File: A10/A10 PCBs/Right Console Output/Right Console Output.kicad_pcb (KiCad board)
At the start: 2 copper layers, 99.7 x 98.4 mm, 78 parts, among them J1 BACKLIGHT, J10 PATCH, J11 PATCH, J12 BACKLIGHT, J13 BACKLIGHT, J14 BACKLIGHT, J15 PATCH, J16 PATCH, J17 BACKLIGHT, J18 BACKLIGHT, J19 BACKLIGHT, J2 BACKLIGHT, J20 5VIN, J21 LOX, J22 12VIN, J23 CABIN_PRES, J24 PWM, J25 PWM, J26 Communication, J27 OXY_REG, J28 RIGHT FUEL, J29 LEFT_FUEL, J3 BACKLIGHT, J30 RIGHT_HYD, J31 LEFT_HYD, J32 Analog, J33 Analog, J34 CABIN_PRES, J35 OXY_REG, J36 LOX, J37 RIGHT_HYD, J38 LEFT_FUEL, J39 RIGHT FUEL, J4 BACKLIGHT, J40 LEFT_HYD, J41 Power, J42 Power, J43 Analog, J44 Analog, J45 Digital, J46 PWM, J47 PWM, J48 Communication, J49 CAUTION_UPPER_DIGIT, J5 BACKLIGHT, J50 CAUTION_UPPER_SEG, J51 CAUTION_LOW_DIGITS, J52 CAUTION_LOWER_SEG, J53 OXY_LED, J54 TACAN_TEST, J55 FORWARD_SEGEMENTS, J56 FORWARD_DIGITS, J6 BACKLIGHT, J7 BACKLIGHT, J8 BACKLIGHT, J9 BACKLIGHT, Q1 IRF1405PBF, U1 USR-ES1, U2 MAX7219-A, U3 MAX7219-B

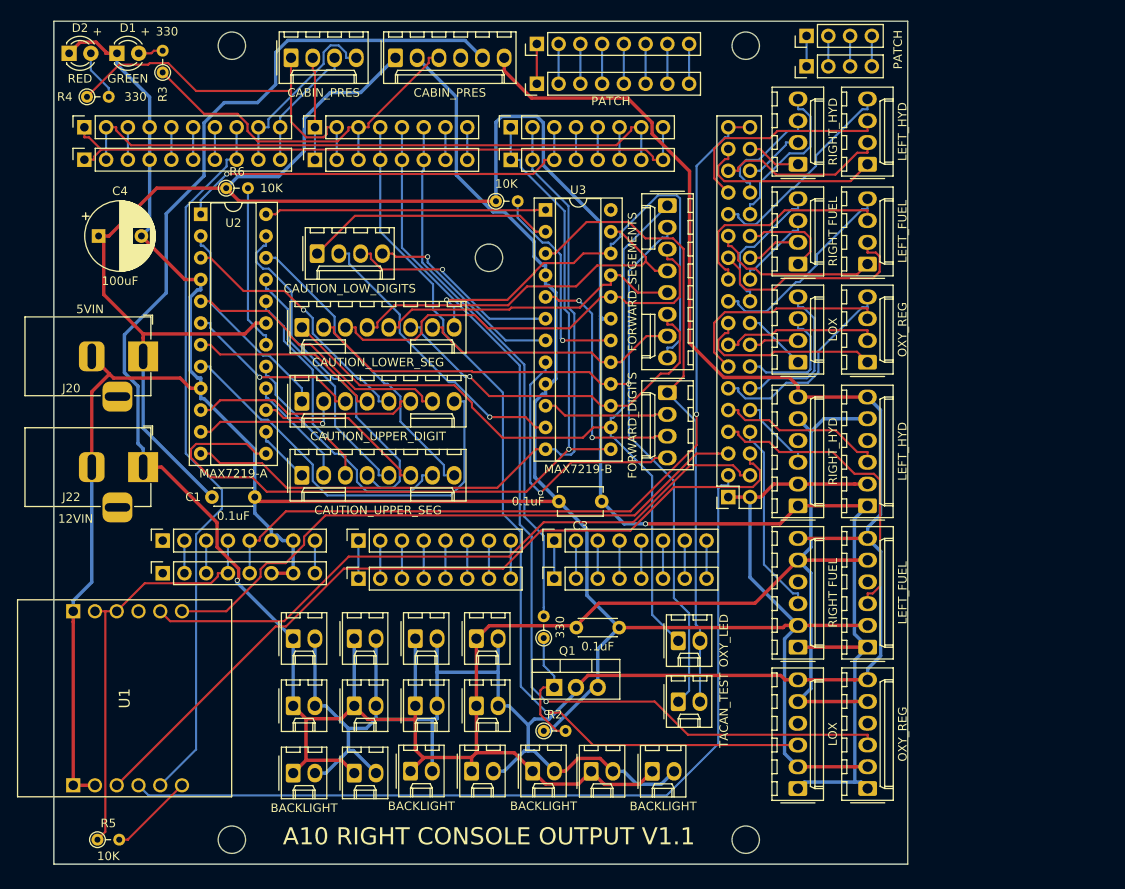
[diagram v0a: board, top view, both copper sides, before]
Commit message: a10 PC
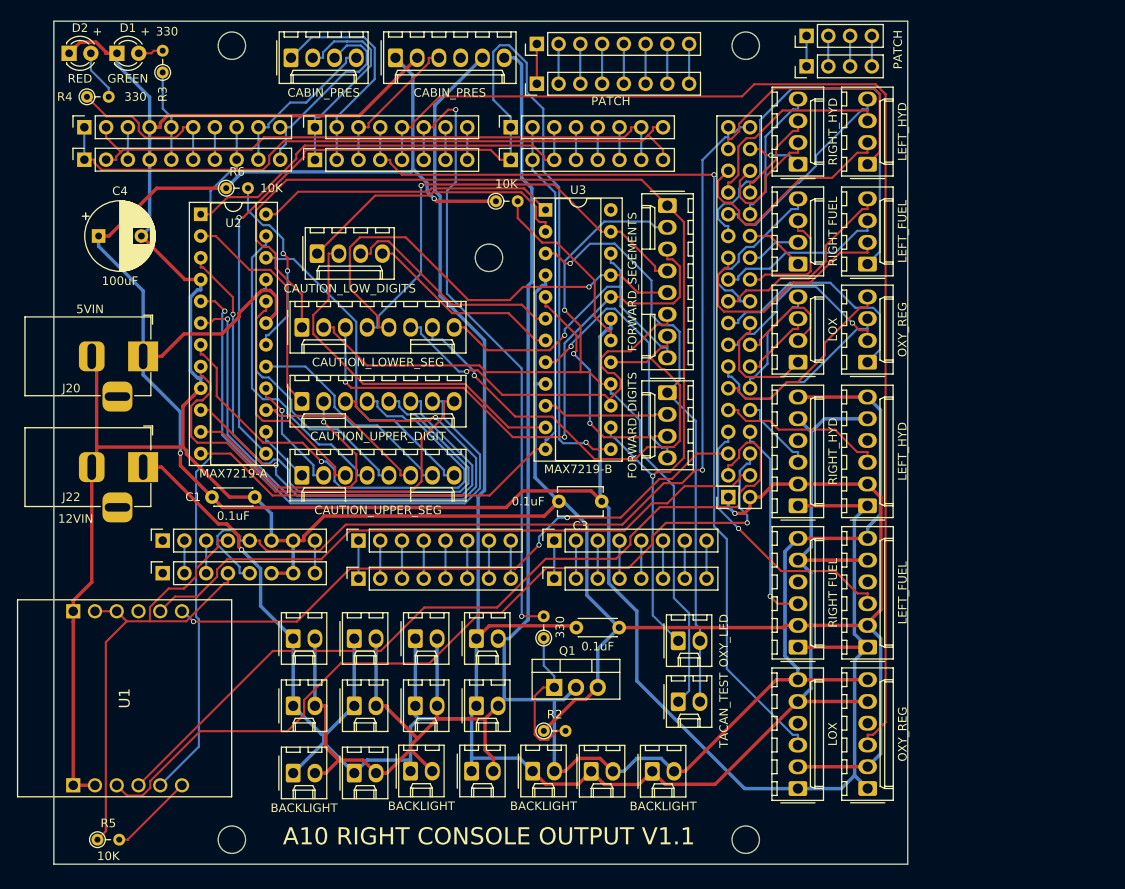
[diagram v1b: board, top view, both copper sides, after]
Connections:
- R3 pad 1: /*5 -> /*13
- R4 pad 1: /*6 -> /*12
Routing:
- net /MAX7219A/DIG_A2: track 21.4 -> 71.6 mm, vias 1 -> 2
- net /MAX7219A/DIG_A4: track 30.3 -> 68.9 mm
- net /MAX7219A/DIG_A3: track 22.5 -> 57.8 mm, vias 0 -> 1
- net /30: track 19.8 -> 53.5 mm
- net /MAX7219A/DIG_A6: track 32.4 -> 65.2 mm, vias 0 -> 1
- net CLK: track 104.3 -> 135.3 mm, vias 1 -> 2
- net /MAX7219A/SEG_A1: track 99.4 -> 130.2 mm, vias 0 -> 1
- net /*5: track 44.8 -> 17.2 mm
- net /MAX7219A/SEG_G1: track 30.7 -> 57.1 mm, vias 0 -> 1
- net /*3: track 114.4 -> 140.3 mm, vias 1 -> 0
- net /MAX7219A/DIG_A5: track 26.6 -> 50.6 mm, vias 0 -> 1
- net +5VD: track 275.9 -> 299.7 mm, vias 1 -> 2
- net +12V: track 320.6 -> 301.1 mm
- net /*6: track 45.1 -> 26.2 mm
- net /MAX7219A/SEG_E1: track 36.9 -> 54.6 mm, vias 0 -> 1
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
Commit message: A10
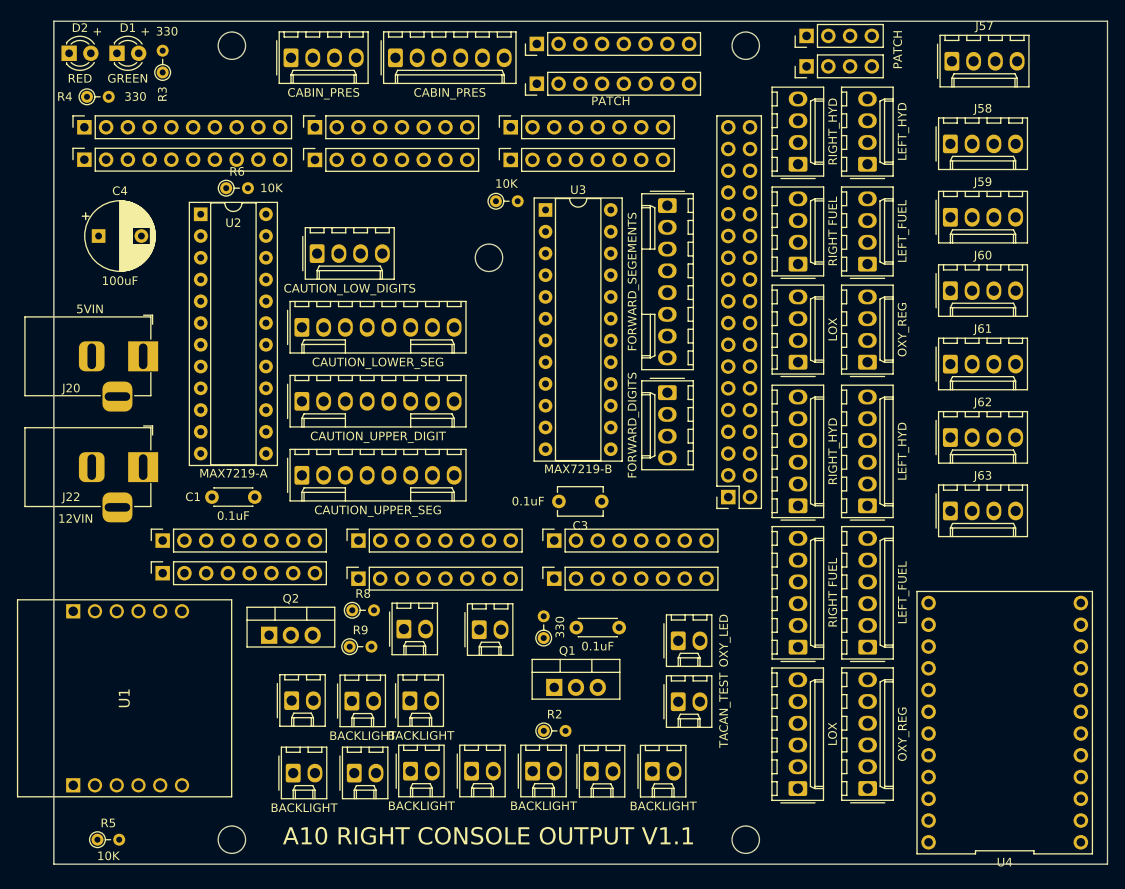
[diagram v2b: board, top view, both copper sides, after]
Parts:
- removed J1, J17, J4: BACKLIGHT, Connector_Molex:Molex_KK-254_AE-6410-02A_1x02_P2.54mm_Vertical
- added J57: CMSP_OLED, Connector_Molex:Molex_KK-254_AE-6410-04A_1x04_P2.54mm_Vertical, F.Cu at (220.1, 41.5)
- added J58: FUEL_OLED, Connector_Molex:Molex_KK-254_AE-6410-04A_1x04_P2.54mm_Vertical, F.Cu at (219.9, 51.1)
- added J59: ILS_OLED, Connector_Molex:Molex_KK-254_AE-6410-04A_1x04_P2.54mm_Vertical, F.Cu at (219.9, 59.7)
- added J60: TACAN_OLED, Connector_Molex:Molex_KK-254_AE-6410-04A_1x04_P2.54mm_Vertical, F.Cu at (219.9, 68.3)
- added J61: SPARE_A_OLED, Connector_Molex:Molex_KK-254_AE-6410-04A_1x04_P2.54mm_Vertical, F.Cu at (219.9, 76.9)
- added J62: SPARE_B_OLED, Connector_Molex:Molex_KK-254_AE-6410-04A_1x04_P2.54mm_Vertical, F.Cu at (219.9, 85.4)
- added J63: SPARE_C_OLED, Connector_Molex:Molex_KK-254_AE-6410-04A_1x04_P2.54mm_Vertical, F.Cu at (219.9, 94.0)
- added Q2: IRF1405PBF, Package_TO_SOT_THT:TO-220-3_Vertical, F.Cu at (140.4, 108.5)
- added R8: 330, Resistor_THT:R_Axial_DIN0204_L3.6mm_D1.6mm_P2.54mm_Vertical, F.Cu at (150.1, 105.6)
- added R9: 10K, Resistor_THT:R_Axial_DIN0204_L3.6mm_D1.6mm_P2.54mm_Vertical, F.Cu at (149.8, 109.8)
- added U4: TCA9548APWR, Footprint Library:DIP-24_TCA9548A, F.Cu at (226.3, 118.7)
- J12, J7: value BACKLIGHT -> FLOODLIGHT
- moved J7 12.3 mm to (156.1, 107.8)
- moved J12 11.6 mm to (164.9, 107.9)
- moved J8 7.29 mm to (150.0, 116.2)
- moved J13 7.29 mm to (156.8, 116.2)
- moved J5 0.64 mm to (143.0, 116.2)
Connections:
- net /*11 renamed D11
- net /RX1/19 renamed D19
- net /RX2/17 renamed D17
- net /SCL/21 renamed D21 SCL
- net /SDA/20 renamed D20 SDA
- net /TX1/18 renamed D18
- J12 pad 2: /BACKLIGHT_-V -> /FLOODLIGHT_-V
- J27 pad 3: /*3 -> unconnected-(J27-Pin_3-Pad3)
- J7 pad 2: /BACKLIGHT_-V -> /FLOODLIGHT_-V
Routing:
- net GND: track 375.8 -> 0.00 mm, vias 1 -> 0
- net +12V: track 301.1 -> 0.00 mm, vias 1 -> 0
- net +5VD: track 299.7 -> 0.00 mm, vias 2 -> 0
- net /BACKLIGHT_-V: track 269.1 -> 0.00 mm
- net /*3: track 140.3 -> 0.00 mm
- net CLK: track 135.3 -> 0.00 mm, vias 2 -> 0
- net /MAX7219A/SEG_A1: track 130.2 -> 0.00 mm, vias 1 -> 0
- net /*4: track 114.7 -> 0.00 mm, vias 1 -> 0
- net +5V: track 113.1 -> 0.00 mm, vias 1 -> 0
- net /MAX7219A/SEG_B1: track 106.1 -> 0.00 mm, vias 1 -> 0
- net SCLK: track 99.1 -> 0.00 mm
- net MOSI: track 98.5 -> 0.00 mm, vias 1 -> 0
- net LOAD: track 83.8 -> 0.00 mm
- net SS: track 81.1 -> 0.00 mm
- net D21 SCL: track 78.5 -> 0.00 mm
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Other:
- board size 99.7 x 98.4 mm -> 123 x 98.4 mm

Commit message: a10
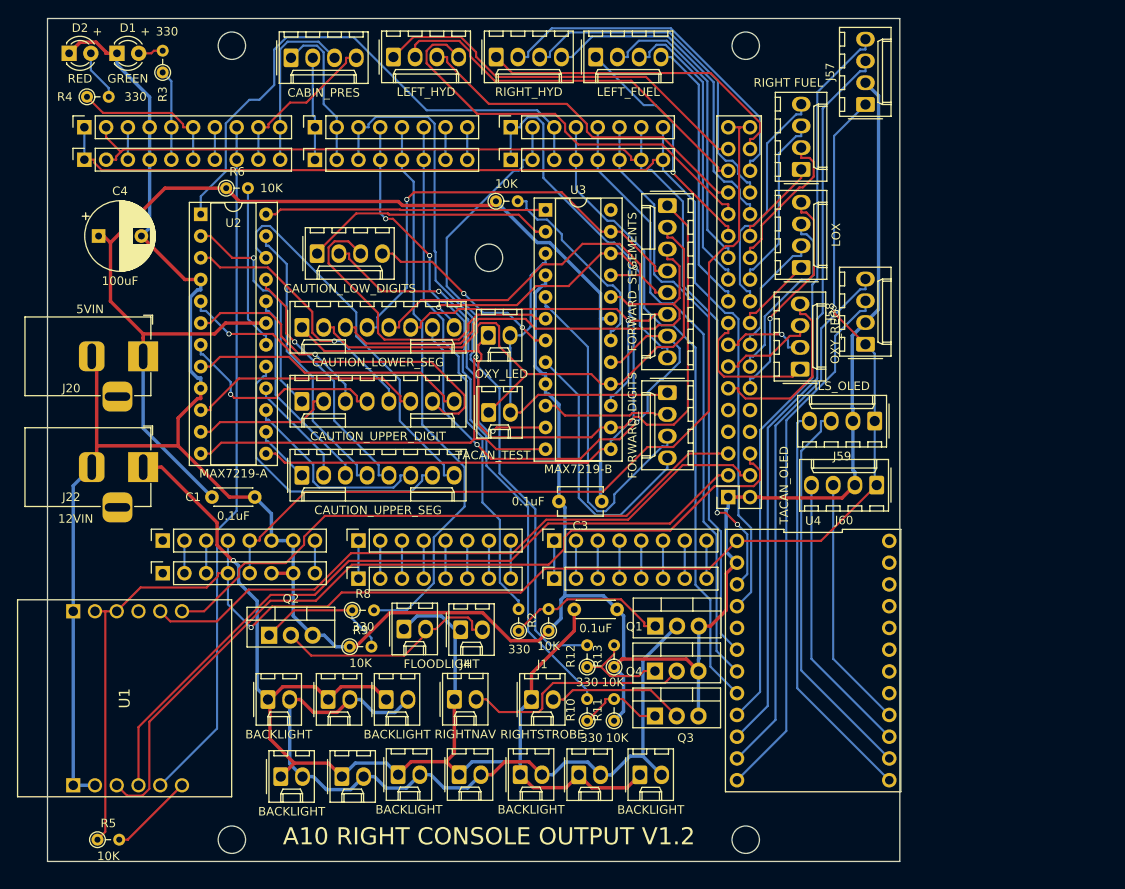
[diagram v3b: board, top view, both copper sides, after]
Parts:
- removed J10, J15: PATCH, Connector_PinHeader_2.54mm:PinHeader_1x04_P2.54mm_Vertical
- removed J11, J16: PATCH, Connector_PinHeader_2.54mm:PinHeader_1x08_P2.54mm_Vertical
- removed J21: LOX, Connector_Molex:Molex_KK-254_AE-6410-06A_1x06_P2.54mm_Vertical
- removed J23: CABIN_PRES, Connector_Molex:Molex_KK-254_AE-6410-06A_1x06_P2.54mm_Vertical
- removed J27: OXY_REG, Connector_Molex:Molex_KK-254_AE-6410-06A_1x06_P2.54mm_Vertical
- removed J28: RIGHT FUEL, Connector_Molex:Molex_KK-254_AE-6410-06A_1x06_P2.54mm_Vertical
- removed J29: LEFT_FUEL, Connector_Molex:Molex_KK-254_AE-6410-06A_1x06_P2.54mm_Vertical
- removed J30: RIGHT_HYD, Connector_Molex:Molex_KK-254_AE-6410-06A_1x06_P2.54mm_Vertical
- removed J31: LEFT_HYD, Connector_Molex:Molex_KK-254_AE-6410-06A_1x06_P2.54mm_Vertical
- removed J61: SPARE_A_OLED, Connector_Molex:Molex_KK-254_AE-6410-04A_1x04_P2.54mm_Vertical
- removed J62: SPARE_B_OLED, Connector_Molex:Molex_KK-254_AE-6410-04A_1x04_P2.54mm_Vertical
- removed J63: SPARE_C_OLED, Connector_Molex:Molex_KK-254_AE-6410-04A_1x04_P2.54mm_Vertical
- added J1: RIGHTSTROBE, Connector_Molex:Molex_KK-254_AE-6410-02A_1x02_P2.54mm_Vertical, F.Cu at (171.0, 116.0)
- added J4: RIGHTNAV, Connector_Molex:Molex_KK-254_AE-6410-02A_1x02_P2.54mm_Vertical, F.Cu at (162.0, 116.0)
- added Q3: IRF1405PBF, Package_TO_SOT_THT:TO-220-3_Vertical, F.Cu at (185.4, 117.9)
- added Q4: IRF1405PBF, Package_TO_SOT_THT:TO-220-3_Vertical, F.Cu at (185.4, 112.7)
- added R10: 330, Resistor_THT:R_Axial_DIN0204_L3.6mm_D1.6mm_P2.54mm_Vertical, F.Cu at (177.5, 118.5)
- added R11: 10K, Resistor_THT:R_Axial_DIN0204_L3.6mm_D1.6mm_P2.54mm_Vertical, F.Cu at (180.7, 118.5)
- added R12: 330, Resistor_THT:R_Axial_DIN0204_L3.6mm_D1.6mm_P2.54mm_Vertical, F.Cu at (177.5, 112.2)
- added R13: 10K, Resistor_THT:R_Axial_DIN0204_L3.6mm_D1.6mm_P2.54mm_Vertical, F.Cu at (180.7, 112.2)
- moved J40 56.8 mm to (154.9, 41.0), turned to 0 degrees
- moved J53 42.0 mm to (166.0, 73.5)
- moved J54 40.4 mm to (166.0, 82.5)
- moved J38 39.9 mm to (178.5, 41.0), turned to 0 degrees
- moved J37 37.4 mm to (166.9, 41.0), turned to 0 degrees
- moved J58 25.4 mm to (210.0, 74.5), turned to 90 degrees
- moved J59 25.4 mm to (211.1, 83.5), turned to 180 degrees
- moved J60 24.3 mm to (211.3, 91.0), turned to 180 degrees
- moved U4 23.5 mm to (203.9, 111.5), turned to -90 degrees
- moved Q1 13.8 mm to (185.5, 107.4)
- moved R2 11.7 mm to (173.0, 108.0), turned to 90 degrees
- moved J57 11.3 mm to (210.0, 46.5), turned to 90 degrees
- moved J36 11.1 mm to (202.5, 65.6)
- moved J39 11.1 mm to (202.5, 54.1)
- moved J35 7.91 mm to (202.4, 77.4)
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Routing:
- net GND: track 0.00 -> 361.2 mm
- net +3V3: track 0.00 -> 183.9 mm, vias 0 -> 2
- net +12V: track 0.00 -> 153.9 mm, vias 0 -> 1
- net +5VD: track 0.00 -> 142.1 mm
- net D21 SCL: track 0.00 -> 134.1 mm
- net D20 SDA: track 0.00 -> 127.8 mm, vias 0 -> 2
- net +5V: track 0.00 -> 101.6 mm
- net MOSI: track 0.00 -> 100.0 mm
- net CLK: track 0.00 -> 94.0 mm
- net /BACKLIGHT_-V: track 0.00 -> 92.7 mm
- net SCLK: track 0.00 -> 87.8 mm
- net /OLED/SC0: track 0.00 -> 85.5 mm
- net /OLED/SD0: track 0.00 -> 85.5 mm
- net /MAX7219A/SEG_A1: track 0.00 -> 85.1 mm
- net /*5: track 0.00 -> 84.7 mm
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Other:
- board size 123 x 98.4 mm -> 99.5 x 98.4 mm
- board text added: "A10 RIGHT CONSOLE OUTPUT V1.2"
- board text removed: "-12 BKLIGHT +12"
- board text removed: "A10 RIGHT CONSOLE OUTPUT V1.1"
- board text removed: "ZERO GND +5V"
